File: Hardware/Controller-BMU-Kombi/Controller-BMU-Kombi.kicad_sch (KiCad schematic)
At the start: 19 parts, among them J1 Conn_01x05_Socket, J2 Conn_01x05_Socket, J3 Conn_01x05_Socket, J4 Conn_01x05_Socket, J5 Conn_01x05_Socket, J6 Conn_01x05_Socket, U2 ESP32_NODEMCU

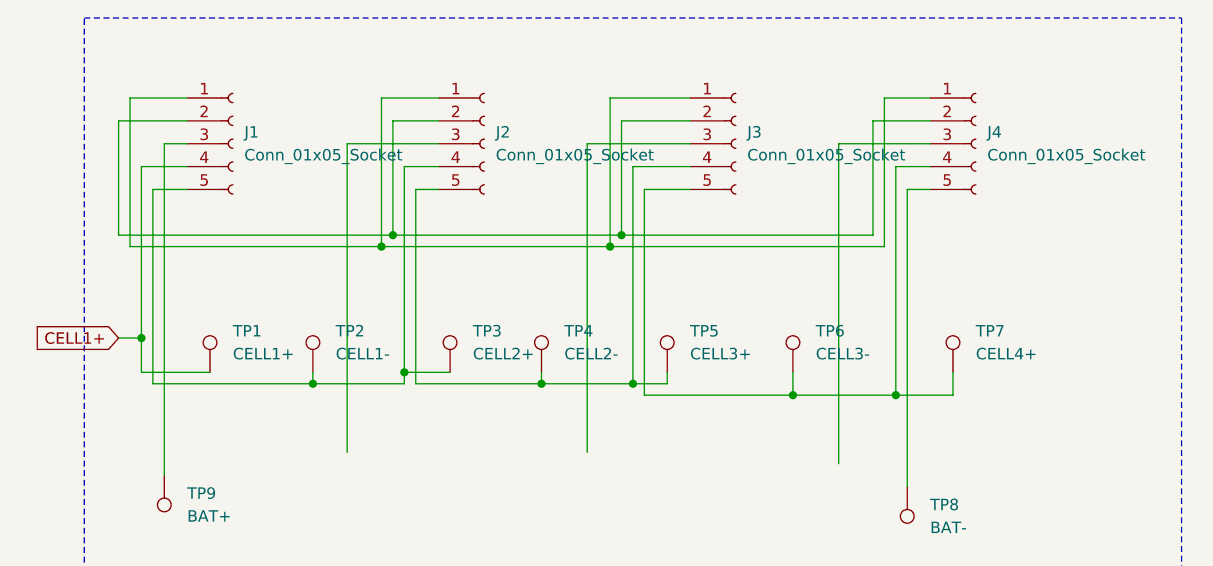
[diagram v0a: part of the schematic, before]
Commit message: synchronizing
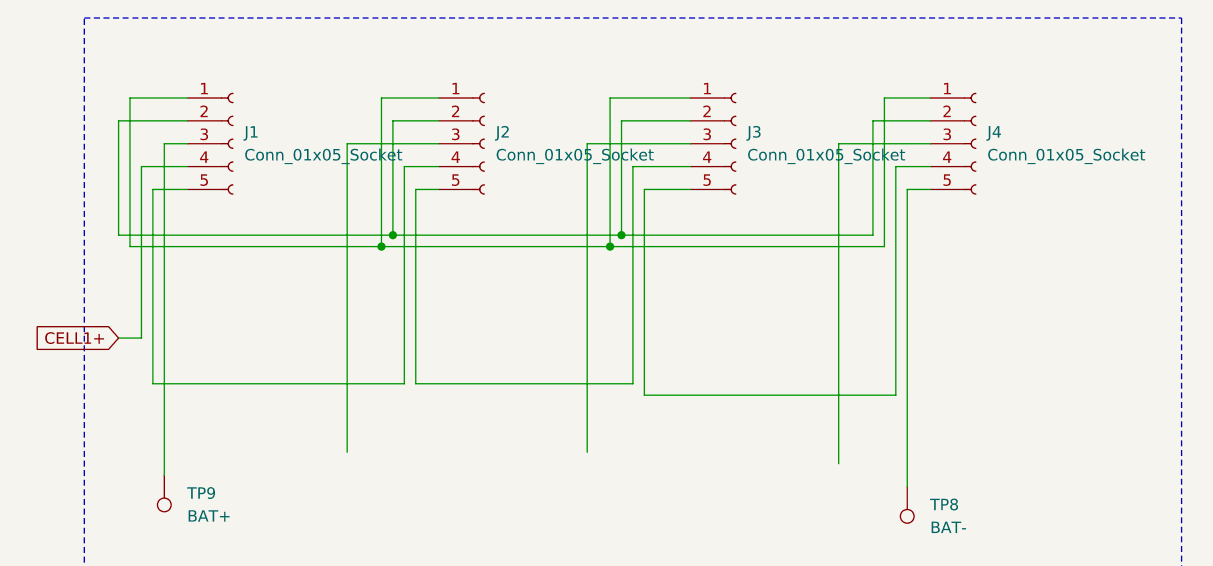
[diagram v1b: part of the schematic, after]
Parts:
- removed TP1: CELL1+, Connector_Pin:Pin_D1.0mm_L10.0mm, symbol Connector:TestPoint
- removed TP2: CELL1-, Connector_Pin:Pin_D1.0mm_L10.0mm, symbol Connector:TestPoint
- removed TP3: CELL2+, Connector_Pin:Pin_D1.0mm_L10.0mm, symbol Connector:TestPoint
- removed TP4: CELL2-, Connector_Pin:Pin_D1.0mm_L10.0mm, symbol Connector:TestPoint
- removed TP5: CELL3+, Connector_Pin:Pin_D1.0mm_L10.0mm, symbol Connector:TestPoint
- removed TP6: CELL3-, Connector_Pin:Pin_D1.0mm_L10.0mm, symbol Connector:TestPoint
- removed TP7: CELL4+, Connector_Pin:Pin_D1.0mm_L10.0mm, symbol Connector:TestPoint
